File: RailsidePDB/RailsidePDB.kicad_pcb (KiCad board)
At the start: 2 copper layers, 64 x 94.5 mm, 129 parts, among them SW1 SW_SPST

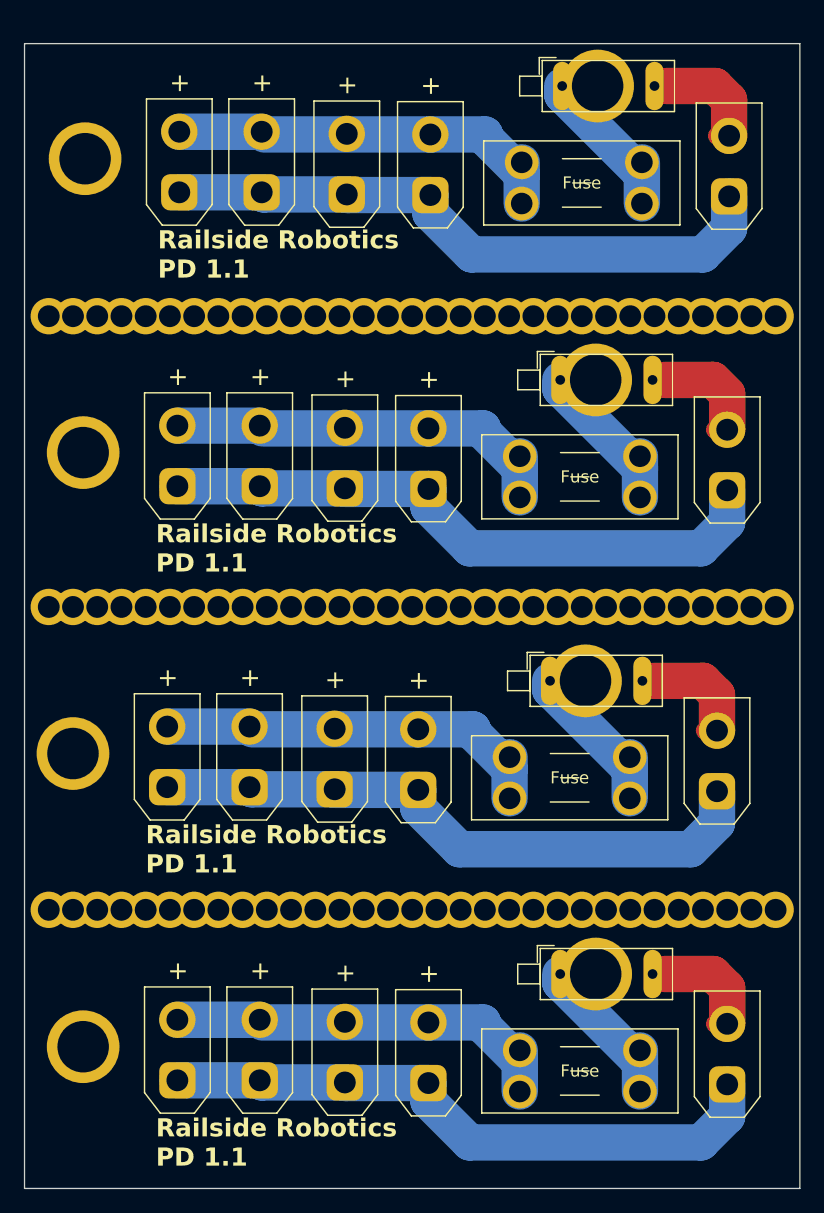
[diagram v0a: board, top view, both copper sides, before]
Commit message: add V3
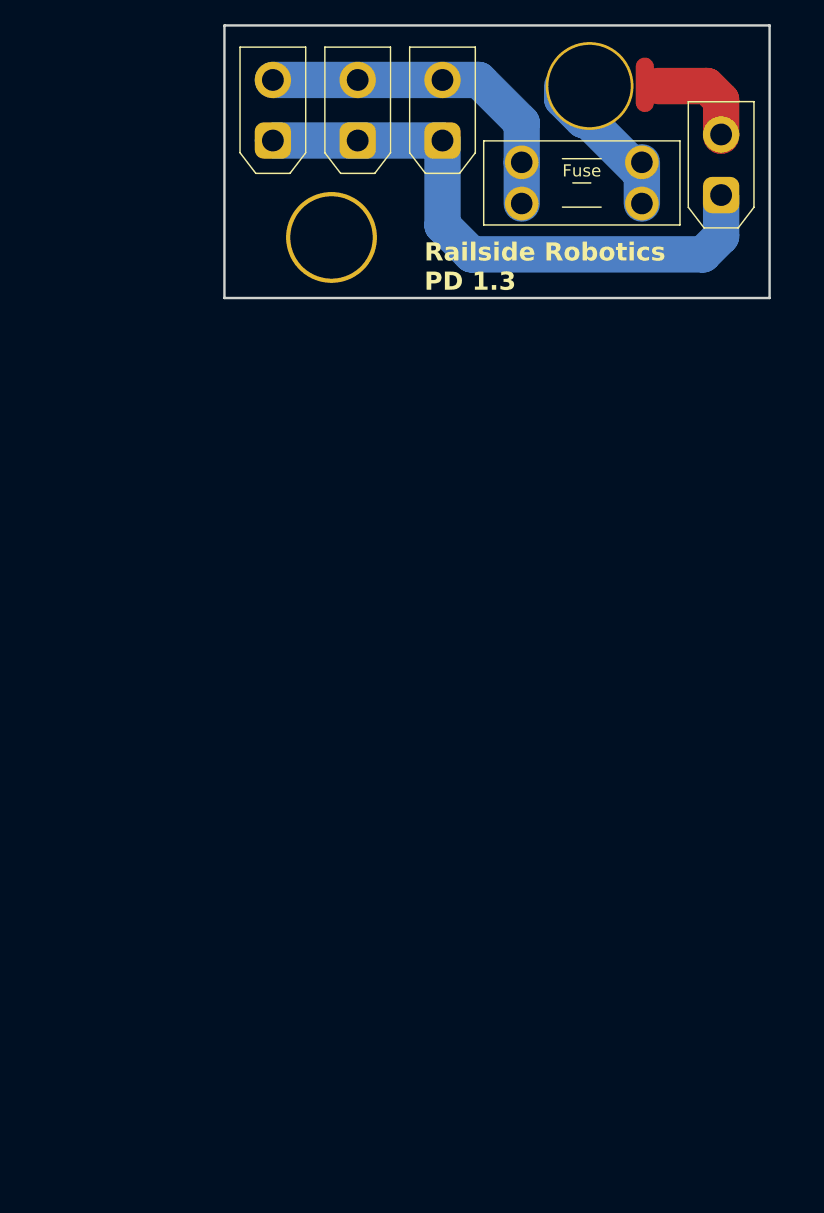
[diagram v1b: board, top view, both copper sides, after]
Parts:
- removed the ? at (53.0, 110.0)
- removed the ? at (65.0, 86.0)
- removed the ? at (55.0, 122.1)
- removed the ? at (89.0, 86.0)
- removed the ? at (57.0, 86.0)
- removed the ? at (61.0, 110.0)
- removed the ? at (109.0, 135.0)
- removed the ? at (97.0, 135.0)
- removed the ? at (105.0, 110.0)
- removed the ? at (87.0, 110.0)
- removed the ? at (103.0, 135.0)
- removed the ? at (59.0, 135.0)
- removed the ? at (55.0, 86.0)
- removed the ? at (59.0, 86.0)
- removed the ? at (113.0, 135.0)
- removed the ? at (69.0, 135.0)
- removed the ? at (55.0, 110.0)
- removed the ? at (101.0, 86.0)
- removed the ? at (65.0, 135.0)
- removed the ? at (91.0, 86.0)
- removed the ? at (87.0, 86.0)
- removed the ? at (105.0, 86.0)
- removed the ? at (95.0, 135.0)
- removed the ? at (69.0, 110.0)
- removed the ? at (85.0, 86.0)
- removed the ? at (93.0, 86.0)
- removed the ? at (67.0, 86.0)
- removed the ? at (97.3, 116.1)
- removed the ? at (109.0, 86.0)
- removed the ? at (57.0, 135.0)
- removed the ? at (57.0, 110.0)
- removed the ? at (91.0, 135.0)
- removed the ? at (113.0, 110.0)
- removed the ? at (73.0, 86.0)
- removed the ? at (75.0, 110.0)
- removed the ? at (79.0, 110.0)
- removed the ? at (71.0, 86.0)
- removed the ? at (101.0, 110.0)
- removed the ? at (97.0, 86.0)
- removed the ? at (55.0, 135.0)
- removed the ? at (99.0, 86.0)
- removed the ? at (111.0, 86.0)
- removed the ? at (69.0, 86.0)
- removed the ? at (71.0, 135.0)
- removed the ? at (91.0, 110.0)
- removed the ? at (55.8, 146.3)
- removed the ? at (93.0, 110.0)
- removed the ? at (75.0, 86.0)
- removed the ? at (89.0, 110.0)
- removed the ? at (73.0, 110.0)
- removed the ? at (97.0, 110.0)
- removed the ? at (95.0, 110.0)
- removed the ? at (103.0, 110.0)
- removed the ? at (101.0, 135.0)
- removed the ? at (107.0, 135.0)
- removed the ? at (98.1, 140.3)
- removed the ? at (63.0, 135.0)
- removed the ? at (107.0, 86.0)
- removed the ? at (111.0, 135.0)
- removed the ? at (56.0, 73.0)
- removed the ? at (77.0, 86.0)
- removed the ? at (63.0, 86.0)
- removed the ? at (103.0, 86.0)
- removed the ? at (99.0, 135.0)
- removed the ? at (85.0, 110.0)
- removed the ? at (107.0, 110.0)
- removed the ? at (87.0, 135.0)
- removed the ? at (83.0, 110.0)
- removed the ? at (67.0, 135.0)
- removed the ? at (59.0, 110.0)
- removed the ? at (105.0, 135.0)
- removed the ? at (93.0, 135.0)
- removed the ? at (98.1, 91.3)
- removed the ? at (83.0, 135.0)
- removed the ? at (95.0, 86.0)
- removed the ? at (83.0, 86.0)
- removed the ? at (73.0, 135.0)
- removed the ? at (65.0, 110.0)
- removed the ? at (71.0, 110.0)
- removed the ? at (61.0, 135.0)
- removed the ? at (109.0, 110.0)
- removed the ? at (55.8, 97.3)
- removed the ? at (81.0, 110.0)
- removed the ? at (99.0, 110.0)
- removed the ? at (53.0, 86.0)
- removed the ? at (81.0, 135.0)
- removed the ? at (79.0, 135.0)
- removed the ? at (67.0, 110.0)
- removed the ? at (89.0, 135.0)
- removed the ? at (111.0, 110.0)
- removed the ? at (53.0, 135.0)
- removed the ? at (77.0, 135.0)
- removed the ? at (113.0, 86.0)
- removed the ? at (61.0, 86.0)
- removed the ? at (75.0, 135.0)
- removed the ? at (81.0, 86.0)
- removed the ? at (63.0, 110.0)
- removed the ? at (85.0, 135.0)
- removed the ? at (79.0, 86.0)
- removed the ? at (77.0, 110.0)
- removed the BT1 at (84.3, 100.3)
- removed the BT1 at (83.5, 125.1)
- removed the BT1 at (84.3, 149.3)
- removed the BT2 at (77.4, 100.2)
- removed the BT2 at (77.4, 149.2)
- removed the BT2 at (76.6, 125.0)
- removed the BT3 at (70.4, 149.1)
- removed the BT3 at (69.6, 124.9)
- removed the BT3 at (70.4, 100.0)
- removed the BT4 at (109.0, 100.4)
- removed the BT4 at (108.2, 125.2)
- removed the BT4 at (109.0, 149.4)
- removed BT5 (x4): Battery, Connector_AMASS:AMASS_XT30UPB-M_1x02_P5.0mm_Vertical
- removed the Fuse at (91.0, 122.4)
- removed the Fuse at (91.9, 97.6)
- removed the Fuse at (91.9, 146.6)
- removed SW1 (x4): SW_SPST, Button_Switch_THT:SW_DIP_SPSTx01_Piano_10.8x4.1mm_W7.62mm_P2.54mm
- added ?: , , F.Cu at (102.2, 66.9)
- added ?: , , F.Cu at (76.3, 79.5)
- moved BT1 4.61 mm to (85.5, 71.5)
- moved BT2 4.54 mm to (78.5, 71.5)
- moved BT3 4.37 mm to (71.5, 71.5)
- moved BT4 0.67 mm to (108.5, 76.0)
- moved ? 0.67 mm to (97.6, 67.0)
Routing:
- net Net-(BT1-+): track 208.9 -> 49.3 mm
- net Net-(BT1--): track 137.2 -> 28.7 mm
- net Net-(SW1-A): track 53.7 -> 13.6 mm
- net Net-(BT4--): track 38.4 -> 8.68 mm
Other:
- board size 64 x 94.5 mm -> 45 x 22.5 mm
- board text added: "Railside Robotics PD 1.3"
- board text removed: "Railside Robotics PD 1.1"
